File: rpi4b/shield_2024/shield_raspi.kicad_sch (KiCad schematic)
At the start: 24 parts, among them J4 Conn_02x20_Odd_Even

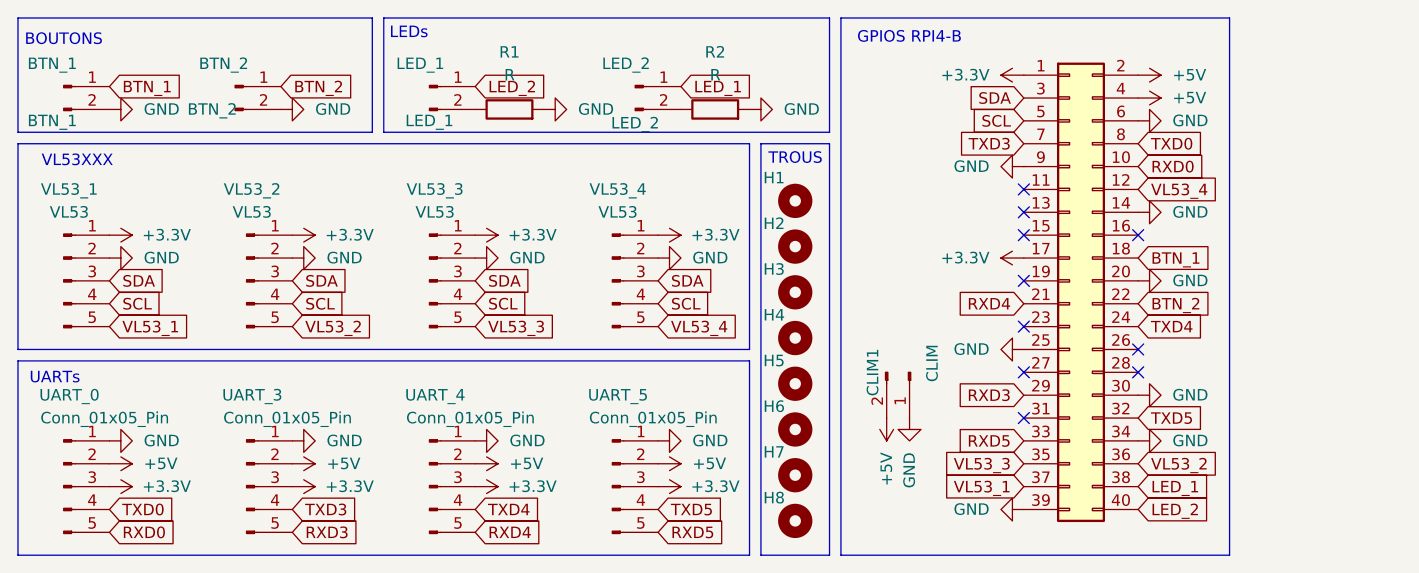
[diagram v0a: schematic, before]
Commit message: WIP le ventillo
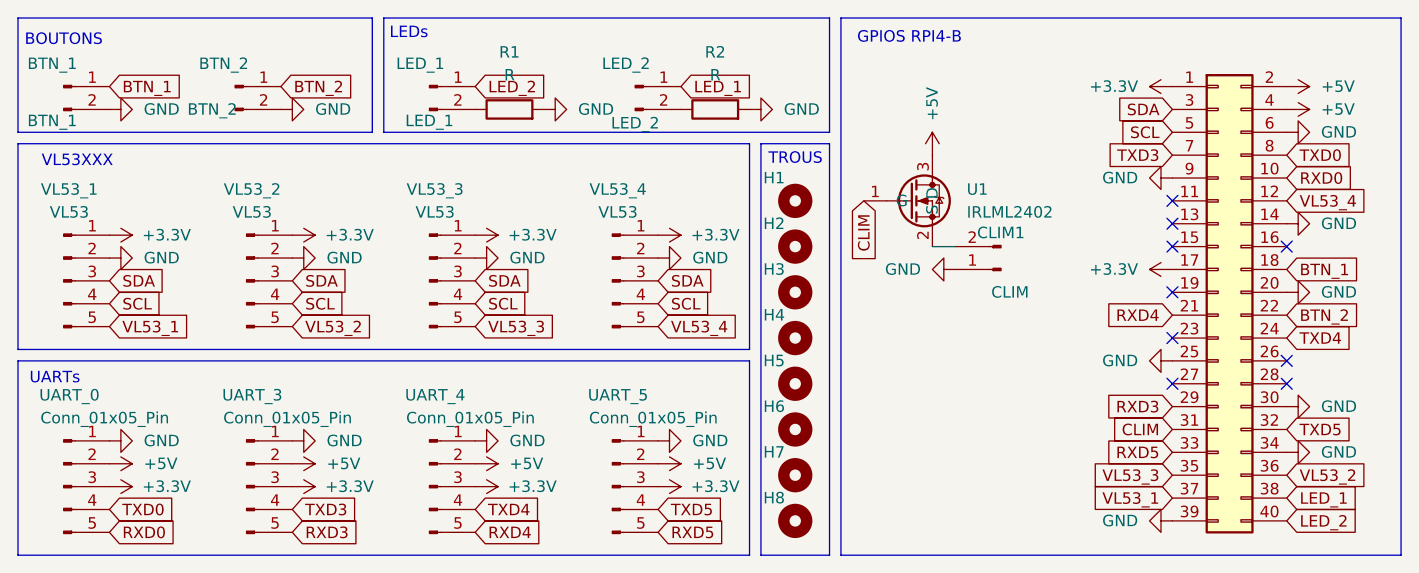
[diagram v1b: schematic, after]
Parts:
- added U1: IRLML2402, myFootprints:SOT-23, symbol mySymbols:IRLML6344
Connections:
- net +5V: now also U1.3 (D); no longer CLIM1.2 (Pin_2)
- net CLIM: now reaches J4.31 (Pin_31)
- net CLIM: now also U1.1 (G)
- new net: CLIM1.2 (Pin_2), U1.2 (S)
- no-connect marks 10 -> 9
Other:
- moved on the sheet: CLIM1
